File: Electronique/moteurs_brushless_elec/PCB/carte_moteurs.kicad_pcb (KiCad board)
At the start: 2 copper layers, 90 x 65 mm, 82 parts, among them J1 CONN_SERIAL, J2 swdio, J3 FAN, K1 Maxon-200142, K2 Maxon-200142, P1 CONN_I2C, P2 CONN_FREE, P3 CONN_CAN, P4 encoder_2, P5 encoder_1, U1 L6235D, U10 Trou-3, U11 Trou-3, U12 B_Plug_5mm, U2 L6235D, U3 stm32f303k8t6, U4 B_Plug_5mm, U5 LM317_SOT223, U6 LM317_SOT223, U7 Trou-3, U8 Trou-3, U9 MCP2562

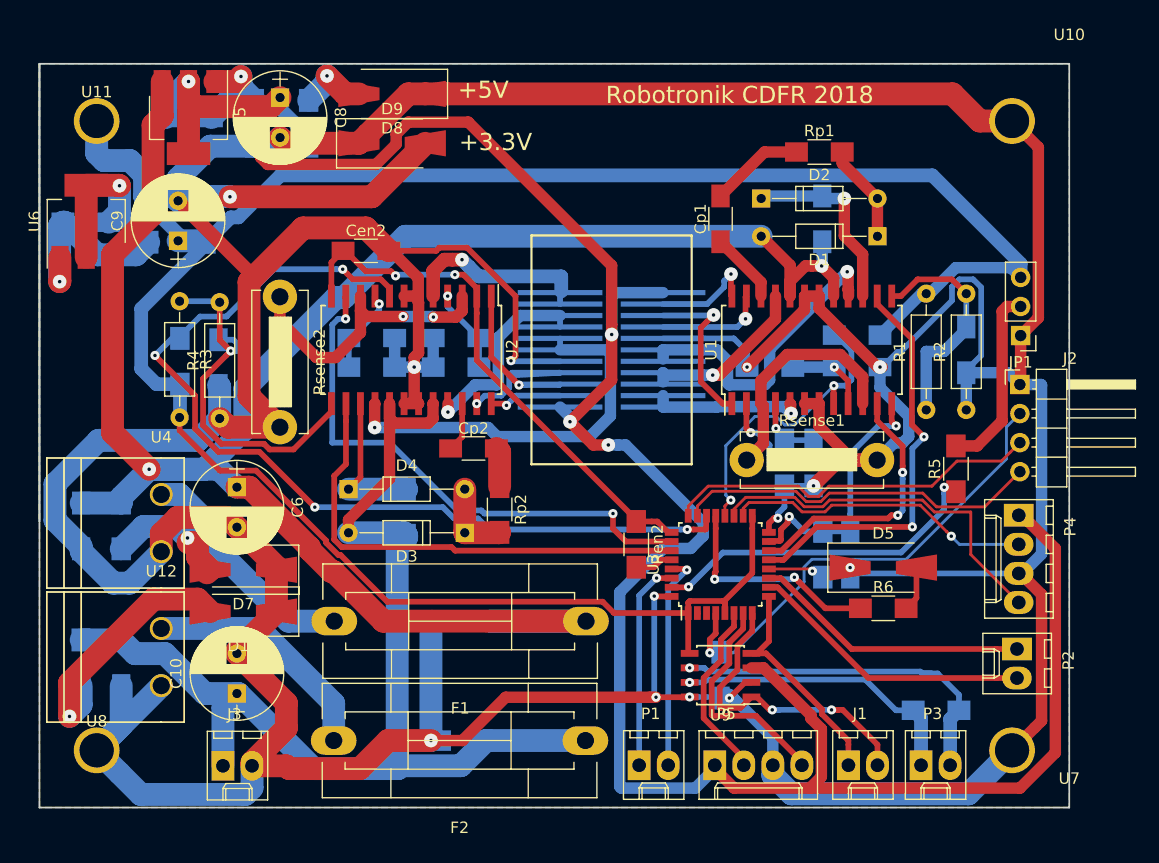
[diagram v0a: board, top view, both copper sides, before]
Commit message: Noms connecteurs brushless
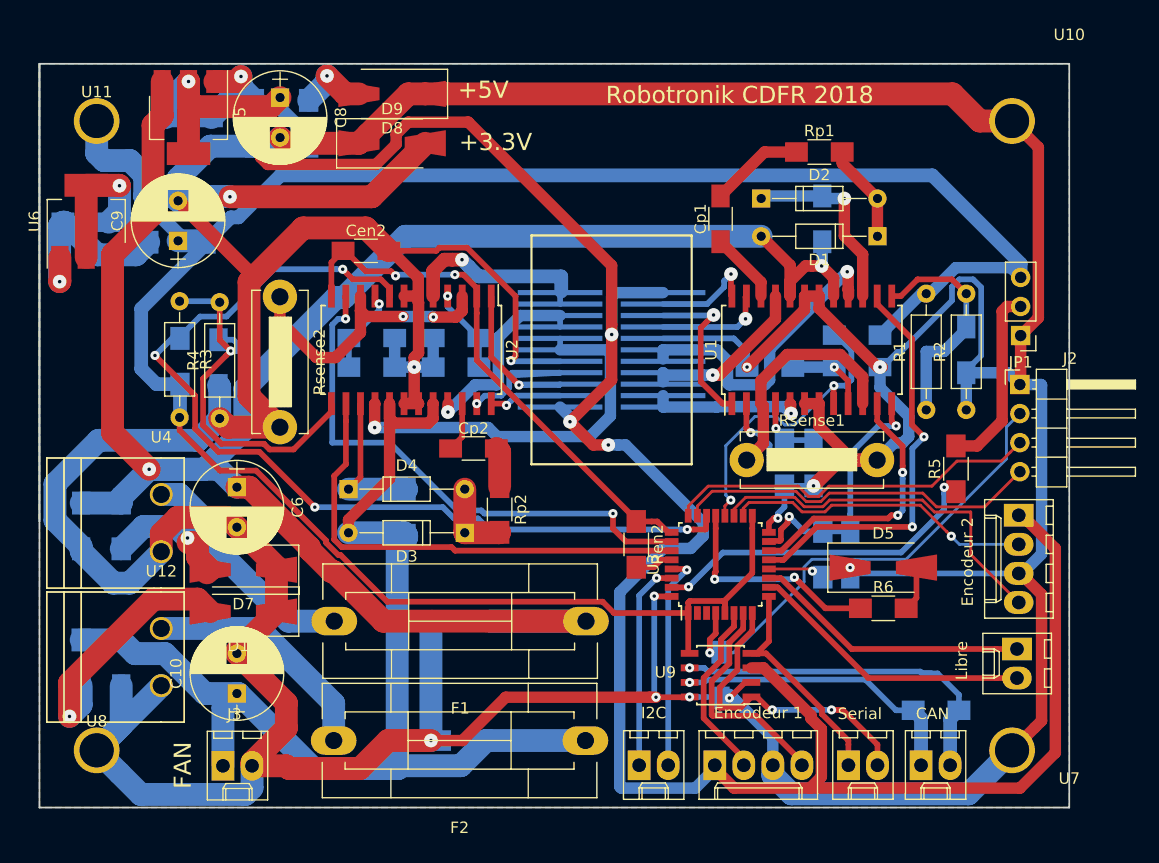
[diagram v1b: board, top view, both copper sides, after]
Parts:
- Encodeur 1: renamed from P5
- Encodeur 2: renamed from P4
- renumbered P3 to CAN, P1 to I2C, P2 to Libre, J1 to Serial
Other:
- board text added: "FAN"
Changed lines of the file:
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@@
   (general
     (links 197)
-    (no_connects 6)
+    (no_connects 0)
     (area 51.6115 80.215 149.459001 152.8396)
     (thickness 1.6)
-    (drawings 14)
+    (drawings 15)
     (tracks 994)
     (zones 0)
@@
   )
   (setup
-    (last_trace_width 0.5)
+    (last_trace_width 1.2)
     (user_trace_width 0.25)
     (user_trace_width 0.5)
@@
     (descr "Connector Headers with Friction Lock, 22-27-2041, http://www.molex.com/pdm_docs/sd/022272021_sd.pdf")
     (tags "connector molex kk_6410 22-27-2041")
-    (fp_text reference P5 (at 1 -4.5) (layer F.SilkS)
+    (fp_text reference "Encodeur 1" (at 3.81 -4.572) (layer F.SilkS)
       (effects (font (size 1 1) (thickness 0.15)))
     )
@@
     (descr "Connector Headers with Friction Lock, 22-27-2021, http://www.molex.com/pdm_docs/sd/022272021_sd.pdf")
     (tags "connector molex kk_6410 22-27-2021")
-    (fp_text reference J1 (at 1 -4.5) (layer F.SilkS)
+    (fp_text reference Serial (at 1 -4.5) (layer F.SilkS)
       (effects (font (size 1 1) (thickness 0.15)))
     )
@@
     (descr "Connector Headers with Friction Lock, 22-27-2021, http://www.molex.com/pdm_docs/sd/022272021_sd.pdf")
     (tags "connector molex kk_6410 22-27-2021")
-    (fp_text reference P1 (at 1 -4.5) (layer F.SilkS)
+    (fp_text reference I2C (at 1.27 -4.572) (layer F.SilkS)
       (effects (font (size 1 1) (thickness 0.15)))
     )
@@
     (descr "Connector Headers with Friction Lock, 22-27-2021, http://www.molex.com/pdm_docs/sd/022272021_sd.pdf")
     (tags "connector molex kk_6410 22-27-2021")
-    (fp_text reference P2 (at 1 -4.5 270) (layer F.SilkS)
+    (fp_text reference Libre (at 1.016 4.826 270) (layer F.SilkS)
       (effects (font (size 1 1) (thickness 0.15)))
     )
@@
     (descr "Connector Headers with Friction Lock, 22-27-2021, http://www.molex.com/pdm_docs/sd/022272021_sd.pdf")
     (tags "connector molex kk_6410 22-27-2021")
-    (fp_text reference P3 (at 1 -4.5) (layer F.SilkS)
+    (fp_text reference CAN (at 1 -4.5) (layer F.SilkS)
       (effects (font (size 1 1) (thickness 0.15)))
     )
@@
     (descr "Connector Headers with Friction Lock, 22-27-2041, http://www.molex.com/pdm_docs/sd/022272021_sd.pdf")
     (tags "connector molex kk_6410 22-27-2041")
-    (fp_text reference P4 (at 1 -4.5 270) (layer F.SilkS)
+    (fp_text reference "Encodeur 2" (at 4.064 4.4704 270) (layer F.SilkS)
       (effects (font (size 1 1) (thickness 0.15)))
     )
@@
     (tags "SOIC 1.27")
     (attr smd)
-    (fp_text reference U9 (at 0 -3.5 180) (layer F.SilkS)
+    (fp_text reference U9 (at 4.826 0.254 180) (layer F.SilkS)
       (effects (font (size 1 1) (thickness 0.15)))
     )
@@
     )
   )
+  (gr_text FAN (at 65.532 146.304 90) (layer F.SilkS)
+    (effects (font (size 1.5 1.5) (thickness 0.3)))
+  )
   (gr_text +3.3V (at 92.8624 91.8464) (layer F.SilkS)
